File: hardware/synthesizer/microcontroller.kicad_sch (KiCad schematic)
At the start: 3 parts, among them J9 Conn_ARM_JTAG_SWD_10, U4 STM32H723VGTx

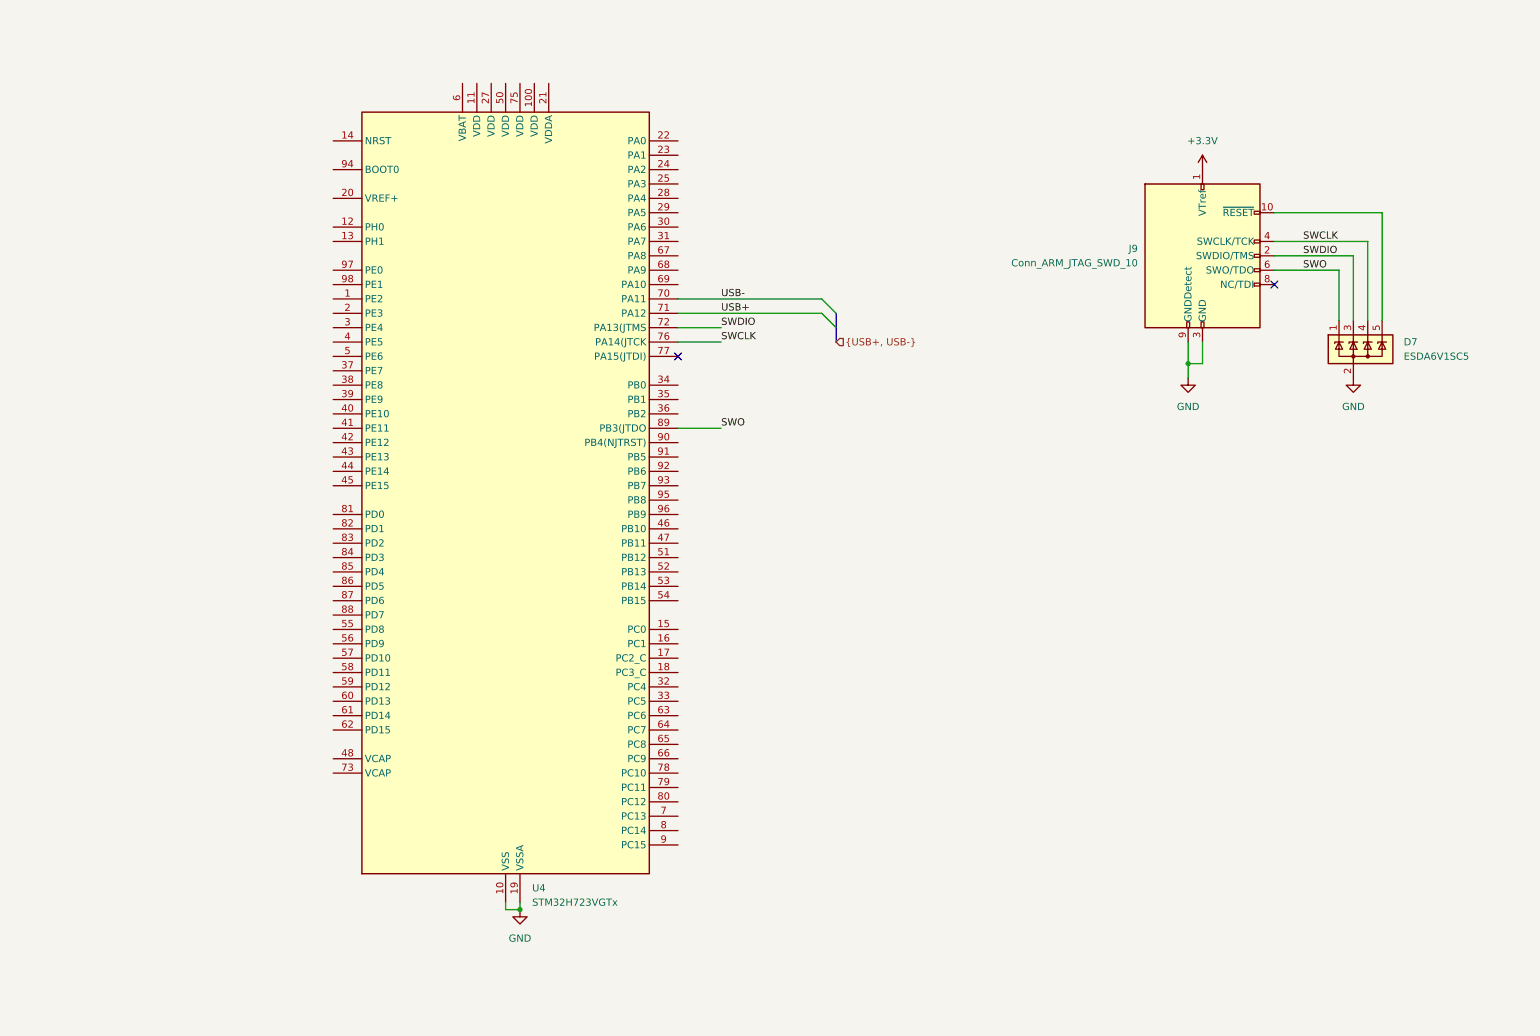
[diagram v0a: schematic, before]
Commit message: work on hardware
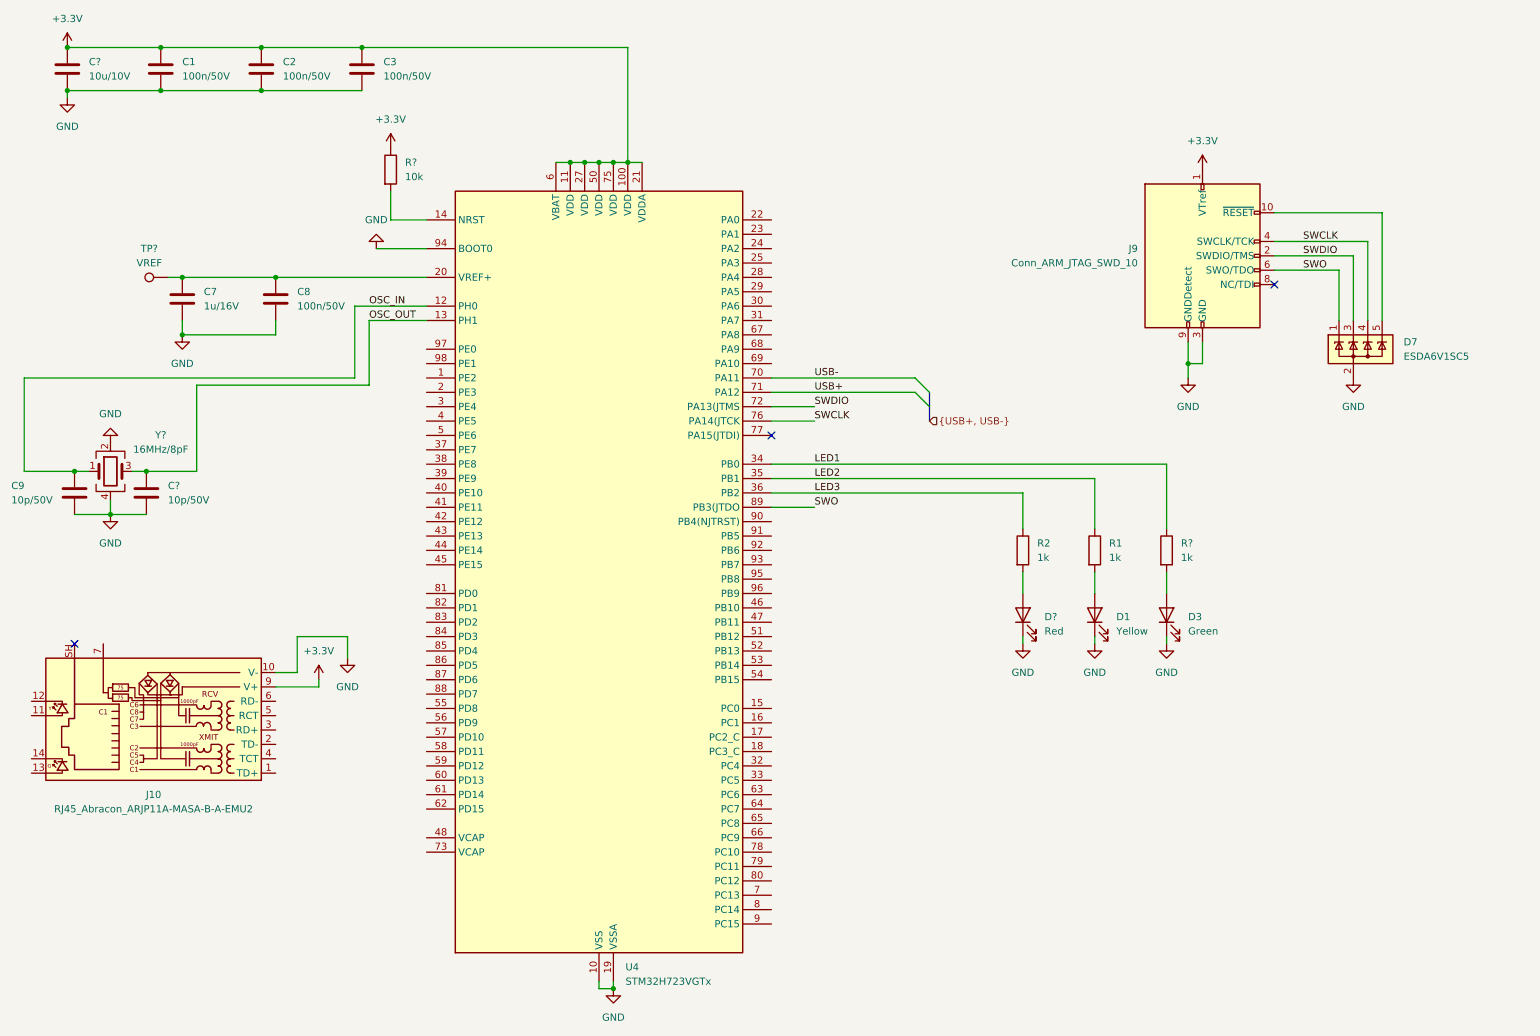
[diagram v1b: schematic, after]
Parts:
- added C1, C2, C3, C8: 100n/50V, symbol Device:C
- added C7: 1u/16V, symbol Device:C
- added C9, C?: 10p/50V, symbol Device:C
- added C?: 10u/10V, symbol Device:C
- added D1: Yellow, symbol Device:LED
- added D3: Green, symbol Device:LED
- added D?: Red, symbol Device:LED
- added J10: RJ45_Abracon_ARJP11A-MASA-B-A-EMU2, Connector_RJ:RJ45_Abracon_ARJP11A-MA_Horizontal, symbol Connector:RJ45_Abracon_ARJP11A-MASA-B-A-EMU2
- added R1, R2, R?: 1k, symbol Device:R
- added R?: 10k, symbol Device:R
- added TP?: VREF, symbol Connector:TestPoint
- added Y?: 16MHz/8pF, symbol Device:Crystal_GND24
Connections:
- net +3.3V: now also U4.100 (VDD), U4.11 (VDD), U4.21 (VDDA), U4.27 (VDD), U4.50 (VDD), U4.6 (VBAT), U4.75 (VDD), C1.1, C2.1, C3.1, C?.1, J10.9 (V+), R?.1
- net GND: now also U4.94 (BOOT0), C1.2, C2.2, C3.2, C7.2, C8.2, C9.2, C?.2, C?.2, D1.1 (K), D3.1 (K), D?.1 (K), J10.10 (V-), Y?.2, Y?.4
- net OSC_IN: now reaches U4.12 (PH0)
- net OSC_IN: now also C9.1, Y?.1
- net OSC_OUT: now reaches U4.13 (PH1)
- net OSC_OUT: now also C?.1, Y?.3
- net at U4.14 (NRST): now also R?.2
- net at U4.20 (VREF+): now also C7.1, C8.1, TP?.1
- net LED1: now reaches U4.34 (PB0)
- net LED1: now also R?.1
- net LED2: now reaches U4.35 (PB1)
- net LED2: now also R1.1
- net LED3: now reaches U4.36 (PB2)
- net LED3: now also R2.1
- new net: D3.2 (A), R?.2
- new net: D1.2 (A), R1.2
- new net: D?.2 (A), R2.2
- no-connect marks 2 -> 3
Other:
- moved on the sheet: U4

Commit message: update synthesizer
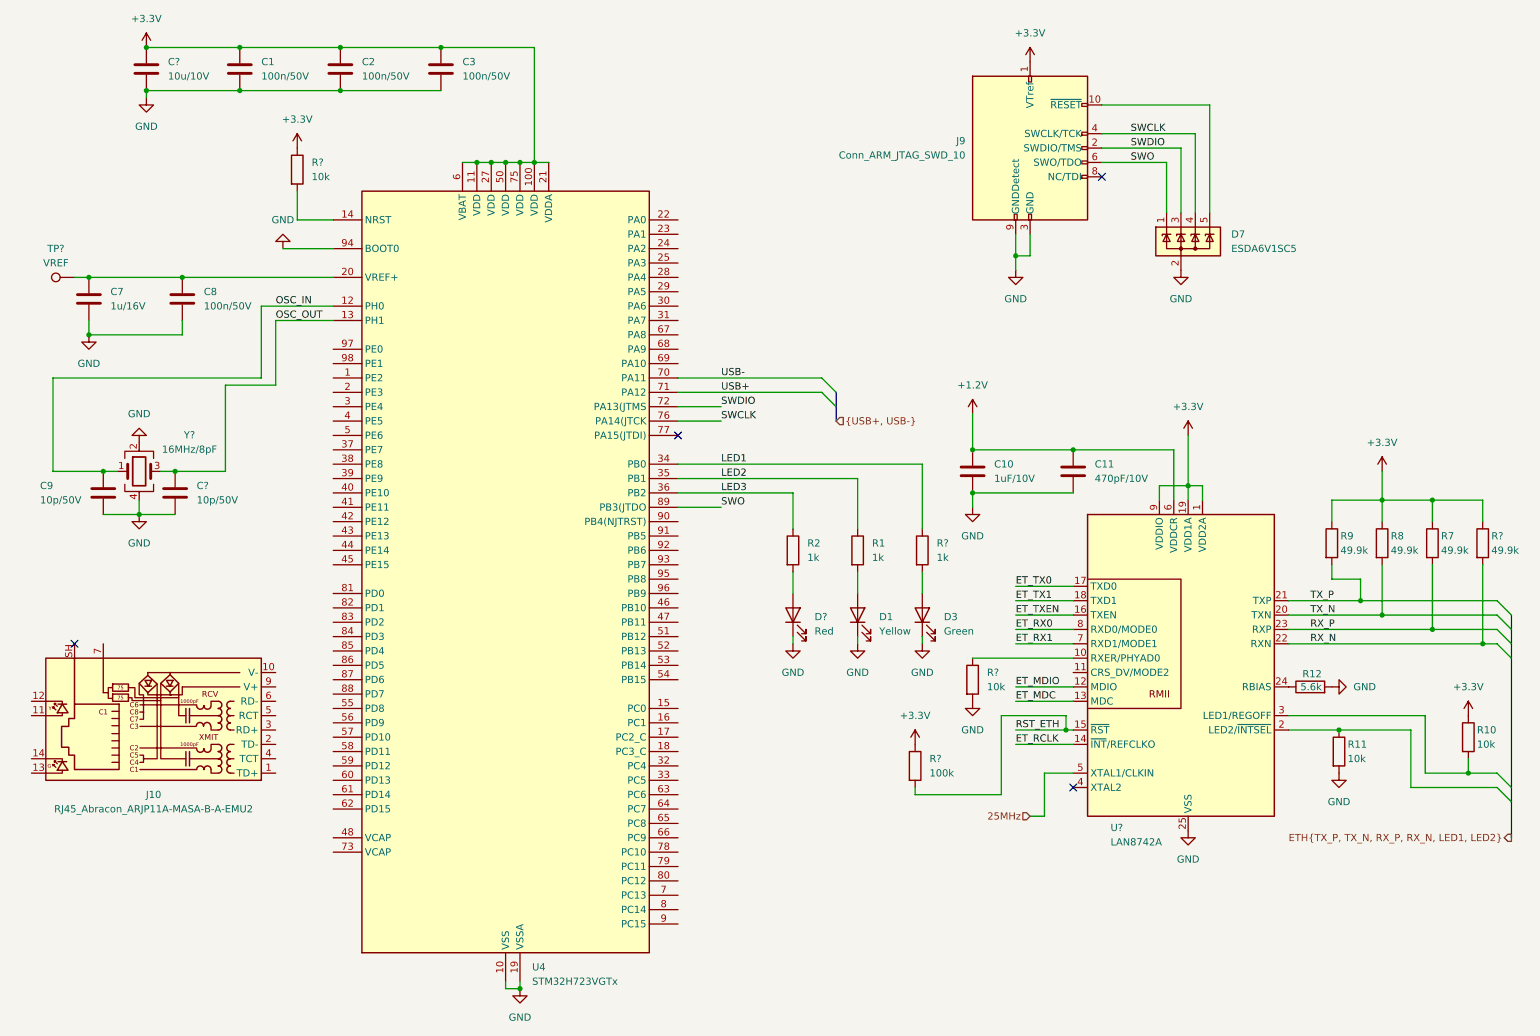
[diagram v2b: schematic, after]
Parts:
- added C10: 1uF/10V, symbol Device:C
- added C11: 470pF/10V, symbol Device:C
- added R10, R11, R?: 10k, symbol Device:R
- added R12: 5.6k, symbol Device:R
- added R7, R8, R9, R?: 49.9k, symbol Device:R
- added R?: 100k, symbol Device:R
- added U?: LAN8742A, Package_DFN_QFN:VQFN-24-1EP_4x4mm_P0.5mm_EP2.5x2.5mm_ThermalVias, symbol Interface_Ethernet:LAN8742A
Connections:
- net +3.3V: now also R10.1, R7.1, R8.1, R9.1, R?.1, R?.1, U?.1 (VDD2A), U?.19 (VDD1A), U?.9 (VDDIO); no longer J10.9 (V+)
- net GND: now also C10.2, C11.2, R11.2, R12.2, R?.2, U?.25 (VSS); no longer J10.10 (V-)
- new net: R?.1, U?.10 (RXER/PHYAD0)
- new net: R11.1, U?.2 (LED2/~{INTSEL})
- new net: R12.1, U?.24 (RBIAS)
- new net: R10.2, U?.3 (LED1/REGOFF)
- new net +1.2V: C10.1, C11.1, U?.6 (VDDCR)
- new net 25MHz: U?.5 (XTAL1/CLKIN)
- new net ET_MDC: U?.13 (MDC)
- new net ET_MDIO: U?.12 (MDIO)
- new net ET_RCLK: U?.14 (~{INT}/REFCLKO)
- new net ET_RX0: U?.8 (RXD0/MODE0)
- new net ET_RX1: U?.7 (RXD1/MODE1)
- new net ET_TX0: U?.17 (TXD0)
- new net ET_TX1: U?.18 (TXD1)
- new net ET_TXEN: U?.16 (TXEN)
- new net RST_ETH: R?.2, U?.15 (~{RST})
- new net RX_N: R?.2, U?.22 (RXN)
- new net RX_P: R7.2, U?.23 (RXP)
- new net TX_N: R8.2, U?.20 (TXN)
- new net TX_P: R9.2, U?.21 (TXP)
- no-connect marks 3 -> 4
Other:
- moved on the sheet: C1, C2, C3, C7, C8, C9, C?, D1, D3, D7, D?, J9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
